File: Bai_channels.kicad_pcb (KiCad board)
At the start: 4 copper layers, 63.5 x 47 mm, 24 parts, among them J2 5019514000, U2 LM7805_TO220, U3 ATmega328-P, U4 ATmega328-P, U5 ATmega328-P

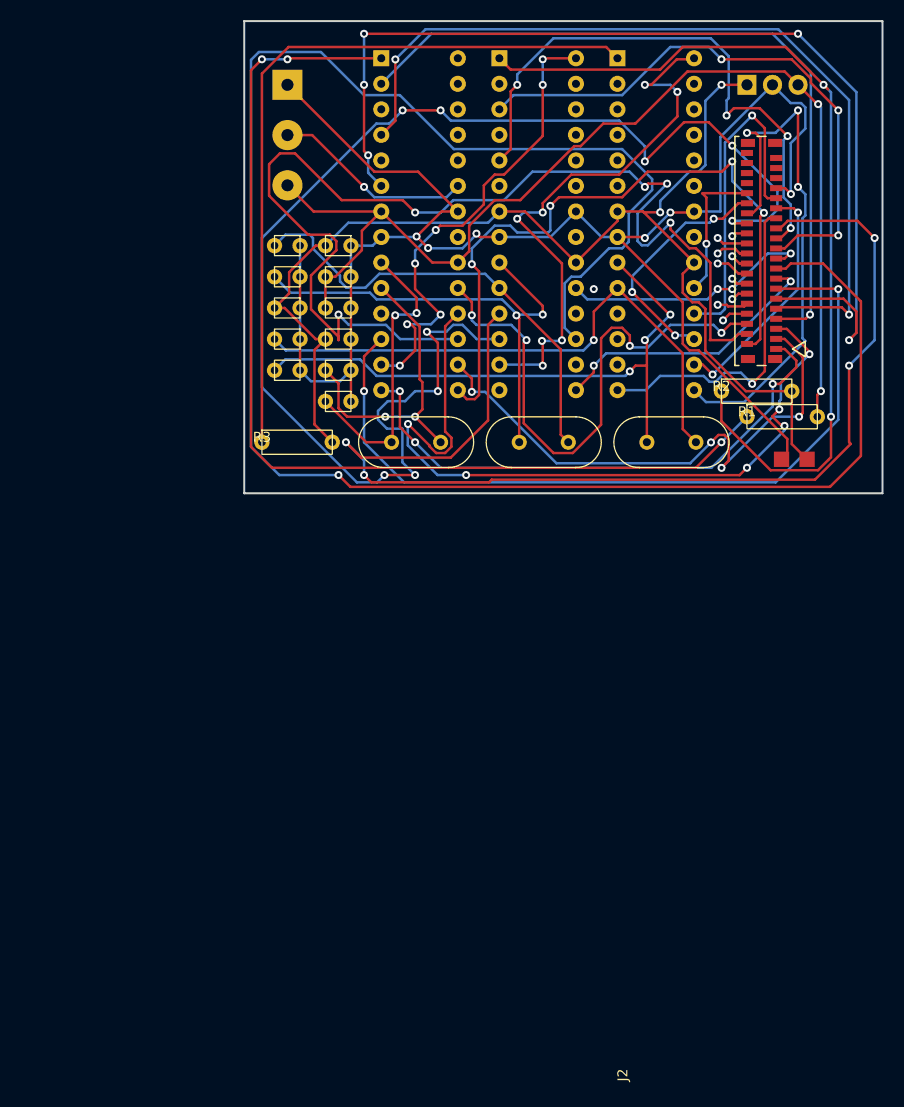
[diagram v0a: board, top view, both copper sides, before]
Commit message: 16 channel
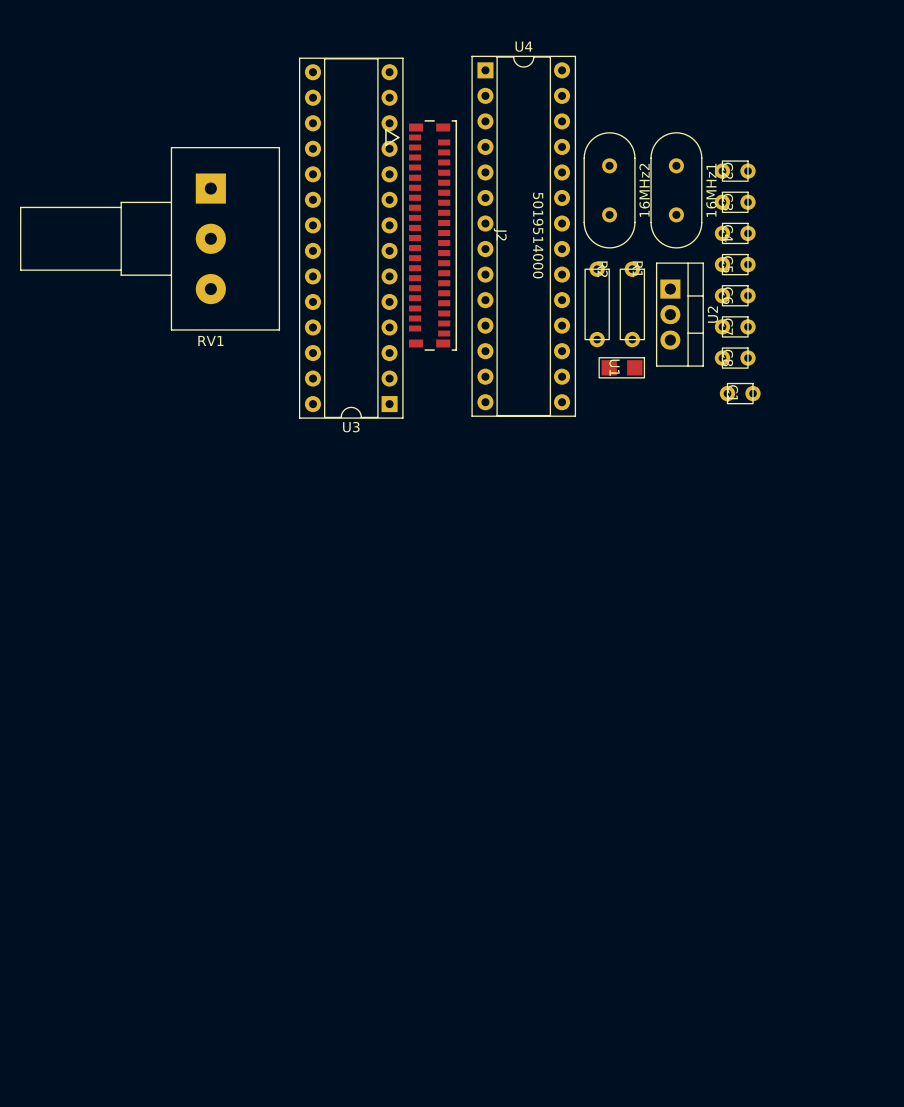
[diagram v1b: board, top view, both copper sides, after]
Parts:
- removed 16MHz3: Crystal, Crystal:Crystal_HC49-4H_Vertical
- removed C10, C11: 22pF, custom:capacitor
- removed C9: 10µF, custom:capacitor
- removed R3: 10kR, custom:R
- removed U5: ATmega328-P, Package_DIP:DIP-28_W7.62mm_Socket
- moved C7 45.3 mm to (157.6, 102.8)
- moved C8 45.3 mm to (157.6, 105.9)
- moved C1 42.6 mm to (158.1, 109.5)
- moved C2 40.9 mm to (157.6, 87.3)
- moved C3 40.9 mm to (157.6, 90.4)
- moved C4 40.9 mm to (157.6, 93.5)
- moved C5 40.9 mm to (157.6, 96.6)
- moved C6 40.9 mm to (157.6, 99.7)
- moved 16MHz1 39.5 mm to (153.0, 86.8), turned to -90 degrees
- moved U3 34.4 mm to (124.5, 110.5), turned to 180 degrees
- moved J2 33.1 mm to (128.4, 93.7), turned to -90 degrees
- moved 16MHz2 28.9 mm to (146.3, 86.8), turned to -90 degrees
- moved U2 21.7 mm to (152.4, 99.1), turned to -90 degrees
- moved U1 21.7 mm to (146.3, 106.9), turned to -90 degrees
- moved R1 18.6 mm to (148.6, 97.1), turned to -90 degrees
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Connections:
- J2 pad 17: Net-(U4-PB3) -> Net-(U1-GND)
- J2 pad 18: Net-(U4-PB4) -> unconnected-(J2-Pad18)
- J2 pad 19: Net-(U4-PB5) -> unconnected-(J2-Pad19)
- J2 pad 20: Net-(U4-PD0) -> unconnected-(J2-Pad20)
- J2 pad 21: Net-(U4-PD1) -> unconnected-(J2-Pad21)
- J2 pad 22: Net-(U4-PD2) -> unconnected-(J2-Pad22)
- J2 pad 23: Net-(U4-PD3) -> unconnected-(J2-Pad23)
- J2 pad 24: Net-(U4-PD4) -> unconnected-(J2-Pad24)
- J2 pad 25: Net-(U4-PD5) -> unconnected-(J2-Pad25)
- J2 pad 26: Net-(U4-PD6) -> unconnected-(J2-Pad26)
- J2 pad 27: Net-(U5-PB0) -> unconnected-(J2-Pad27)
- J2 pad 28: Net-(U5-PB1) -> unconnected-(J2-Pad28)
- J2 pad 29: Net-(U5-PB2) -> unconnected-(J2-Pad29)
- J2 pad 30: Net-(U5-PB3) -> unconnected-(J2-Pad30)
- J2 pad 31: Net-(U5-PB4) -> unconnected-(J2-Pad31)
- J2 pad 32: Net-(U5-PB5) -> unconnected-(J2-Pad32)
- J2 pad 33: Net-(U1-GND) -> unconnected-(J2-Pad33)
- U4 pad 11: Net-(U4-PD5) -> unconnected-(U4-PD5-Pad11)
- U4 pad 12: Net-(U4-PD6) -> unconnected-(U4-PD6-Pad12)
- U4 pad 13: Net-(U4-PD7) -> unconnected-(U4-PD7-Pad13)
- U4 pad 17: Net-(U4-PB3) -> unconnected-(U4-PB3-Pad17)
- U4 pad 18: Net-(U4-PB4) -> unconnected-(U4-PB4-Pad18)
- U4 pad 19: Net-(U4-PB5) -> unconnected-(U4-PB5-Pad19)
- U4 pad 2: Net-(U4-PD0) -> unconnected-(U4-PD0-Pad2)
- U4 pad 3: Net-(U4-PD1) -> unconnected-(U4-PD1-Pad3)
- U4 pad 4: Net-(U4-PD2) -> unconnected-(U4-PD2-Pad4)
- U4 pad 5: Net-(U4-PD3) -> unconnected-(U4-PD3-Pad5)
- U4 pad 6: Net-(U4-PD4) -> unconnected-(U4-PD4-Pad6)
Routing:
- net Net-(U4-PB3): track 194.4 -> 0.00 mm, vias 1 -> 0
- net Net-(U1-GND): track 163.8 -> 0.00 mm, vias 6 -> 0
- net Net-(U4-PD6): track 136.7 -> 0.00 mm, vias 9 -> 0
- net Net-(U1-VCC): track 119.9 -> 0.00 mm, vias 2 -> 0
- net Net-(U4-PD5): track 114.1 -> 0.00 mm, vias 4 -> 0
- net Net-(U3-PB3): track 113.1 -> 0.00 mm, vias 5 -> 0
- net Net-(U2-VO): track 110.4 -> 0.00 mm, vias 2 -> 0
- net Net-(U3-PD4): track 103.9 -> 0.00 mm, vias 5 -> 0
- net Net-(U3-~{RESET}/PC6): track 103.2 -> 0.00 mm, vias 3 -> 0
- net Net-(U4-~{RESET}/PC6): track 89.7 -> 0.00 mm, vias 2 -> 0
- net Net-(U3-PD2): track 86.4 -> 0.00 mm, vias 2 -> 0
- net Net-(U3-PD6): track 81.6 -> 0.00 mm, vias 2 -> 0
- net Net-(U3-PB4): track 76.8 -> 0.00 mm, vias 6 -> 0
- net Net-(U3-PD0): track 74.1 -> 0.00 mm, vias 1 -> 0
- net Net-(U5-~{RESET}/PC6): track 73.6 -> 0.00 mm
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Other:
- board outline removed
